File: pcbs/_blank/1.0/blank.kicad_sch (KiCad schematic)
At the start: 4 parts

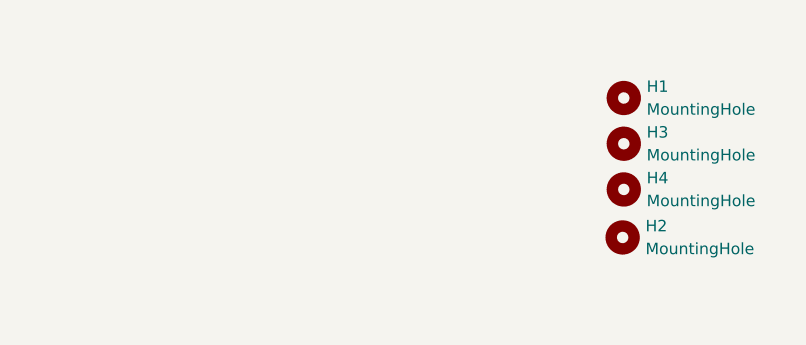
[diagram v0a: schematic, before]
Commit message: Staging
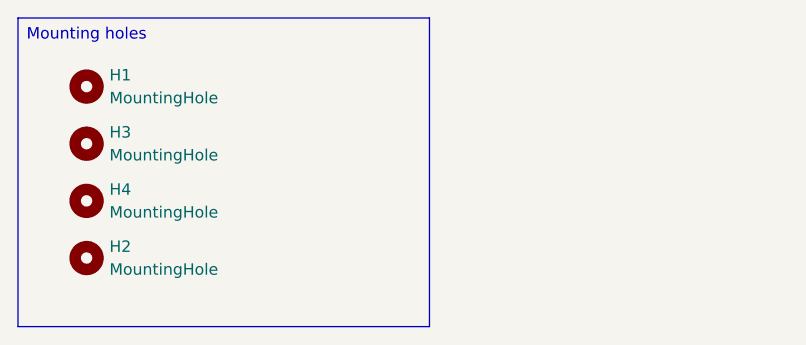
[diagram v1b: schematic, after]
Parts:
- H1, H2, H3, H4: footprint MountingHole:MountingHole_3.2mm_M3_DIN965_Pad_TopOnly -> MountingHole:MountingHole_3.2mm_M3_DIN965_Pad_TopBottom
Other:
- moved on the sheet: H1, H2, H3, H4
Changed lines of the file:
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@@
 (kicad_sch
-	(version 20231120)
+	(version 20250114)
 	(generator "eeschema")
-	(generator_version "8.0")
+	(generator_version "9.0")
 	(paper "A2")
-	(symbol
-		(lib_id "Mechanical:MountingHole")
-		(at 82.55 34.29 0)
+	(text_box "Mounting holes"
+		(exclude_from_sim no)
+		(at 15.24 15.24 0)
+		(size 45.72 34.29)
+		(margins 0.9525 0.9525 0.9525 0.9525)
+		(stroke
+			(width 0)
+			(type solid)
+		)
+		(fill
+			(type none)
+		)
+		(effects
+			(font
+				(size 1.27 1.27)
+			)
+			(justify left top)
+		)
+	)
+	(symbol
+		(lib_id "Mechanical:MountingHole")
+		(at 22.86 35.56 0)
 		(unit 1)
 		(exclude_from_sim no)
@@
 		(fields_autoplaced yes)
 		(property "Reference" "H4"
-			(at 85.09 33.0199 0)
-			(effects
-				(font
-					(size 1.27 1.27)
-				)
-				(justify left)
-			)
-		)
-		(property "Value" "MountingHole"
-			(at 85.09 35.5599 0)
-			(effects
-				(font
-					(size 1.27 1.27)
-				)
-				(justify left)
-			)
-		)
-		(property "Footprint" "MountingHole:MountingHole_3.2mm_M3_DIN965_Pad_TopOnly"
-			(at 82.55 34.29 0)
-			(effects
-				(font
-					(size 1.27 1.27)
-				)
-				(hide yes)
-			)
-		)
-		(property "Datasheet" "~"
-			(at 82.55 34.29 0)
-			(effects
-				(font
-					(size 1.27 1.27)
-				)
-				(hide yes)
-			)
-		)
-		(property "Description" ""
-			(at 82.55 34.29 0)
+			(at 25.4 34.2899 0)
+			(effects
+				(font
+					(size 1.27 1.27)
+				)
+				(justify left)
+			)
+		)
+		(property "Value" "MountingHole"
+			(at 25.4 36.8299 0)
+			(effects
+				(font
+					(size 1.27 1.27)
+				)
+				(justify left)
+			)
+		)
+		(property "Footprint" "MountingHole:MountingHole_3.2mm_M3_DIN965_Pad_TopBottom"
+			(at 22.86 35.56 0)
+			(effects
+				(font
+					(size 1.27 1.27)
+				)
+				(hide yes)
+			)
+		)
+		(property "Datasheet" "~"
+			(at 22.86 35.56 0)
+			(effects
+				(font
+					(size 1.27 1.27)
+				)
+				(hide yes)
+			)
+		)
+		(property "Description" ""
+			(at 22.86 35.56 0)
 			(effects
 				(font
@@
 	(symbol
 		(lib_id "Mechanical:MountingHole")
-		(at 82.55 29.21 0)
+		(at 22.86 29.21 0)
 		(unit 1)
 		(exclude_from_sim no)
@@
 		(fields_autoplaced yes)
 		(property "Reference" "H3"
-			(at 85.09 27.9399 0)
-			(effects
-				(font
-					(size 1.27 1.27)
-				)
-				(justify left)
-			)
-		)
-		(property "Value" "MountingHole"
-			(at 85.09 30.4799 0)
-			(effects
-				(font
-					(size 1.27 1.27)
-				)
-				(justify left)
-			)
-		)
-		(property "Footprint" "MountingHole:MountingHole_3.2mm_M3_DIN965_Pad_TopOnly"
-			(at 82.55 29.21 0)
-			(effects
-				(font
-					(size 1.27 1.27)
-				)
-				(hide yes)
-			)
-		)
-		(property "Datasheet" "~"
-			(at 82.55 29.21 0)
-			(effects
-				(font
-					(size 1.27 1.27)
-				)
-				(hide yes)
-			)
-		)
-		(property "Description" ""
-			(at 82.55 29.21 0)
+			(at 25.4 27.9399 0)
+			(effects
+				(font
+					(size 1.27 1.27)
+				)
+				(justify left)
+			)
+		)
+		(property "Value" "MountingHole"
+			(at 25.4 30.4799 0)
+			(effects
+				(font
+					(size 1.27 1.27)
+				)
+				(justify left)
+			)
+		)
+		(property "Footprint" "MountingHole:MountingHole_3.2mm_M3_DIN965_Pad_TopBottom"
+			(at 22.86 29.21 0)
+			(effects
+				(font
+					(size 1.27 1.27)
+				)
+				(hide yes)
+			)
+		)
+		(property "Datasheet" "~"
+			(at 22.86 29.21 0)
+			(effects
+				(font
+					(size 1.27 1.27)
+				)
+				(hide yes)
+			)
+		)
+		(property "Description" ""
+			(at 22.86 29.21 0)
 			(effects
 				(font
@@
 	(symbol
 		(lib_id "Mechanical:MountingHole")
-		(at 82.55 24.13 0)
+		(at 22.86 22.86 0)
 		(unit 1)
 		(exclude_from_sim no)
@@
 		(fields_autoplaced yes)
 		(property "Reference" "H1"
-			(at 85.09 22.8599 0)
-			(effects
-				(font
-					(size 1.27 1.27)
-				)
-				(justify left)
-			)
-		)
-		(property "Value" "MountingHole"
-			(at 85.09 25.3999 0)
-			(effects
-				(font
-					(size 1.27 1.27)
-				)
-				(justify left)
-			)
-		)
-		(property "Footprint" "MountingHole:MountingHole_3.2mm_M3_DIN965_Pad_TopOnly"
-			(at 82.55 24.13 0)
-			(effects
-				(font
-					(size 1.27 1.27)
-				)
-				(hide yes)
-			)
-		)
-		(property "Datasheet" "~"
-			(at 82.55 24.13 0)
-			(effects
-				(font
-					(size 1.27 1.27)
-				)
-				(hide yes)
-			)
-		)
-		(property "Description" ""
-			(at 82.55 24.13 0)
+			(at 25.4 21.5899 0)
+			(effects
+				(font
+					(size 1.27 1.27)
+				)
+				(justify left)
+			)
+		)
+		(property "Value" "MountingHole"
+			(at 25.4 24.1299 0)
+			(effects
+				(font
+					(size 1.27 1.27)
+				)
+				(justify left)
+			)
+		)
+		(property "Footprint" "MountingHole:MountingHole_3.2mm_M3_DIN965_Pad_TopBottom"
+			(at 22.86 22.86 0)
+			(effects
+				(font
+					(size 1.27 1.27)
+				)
+				(hide yes)
+			)
+		)
+		(property "Datasheet" "~"
+			(at 22.86 22.86 0)
+			(effects
+				(font
+					(size 1.27 1.27)
+				)
+				(hide yes)
+			)
+		)
+		(property "Description" ""
+			(at 22.86 22.86 0)
 			(effects
 				(font
@@
 	(symbol
 		(lib_id "Mechanical:MountingHole")
-		(at 82.423 39.624 0)
+		(at 22.86 41.91 0)
 		(unit 1)
 		(exclude_from_sim no)
@@
 		(fields_autoplaced yes)
 		(property "Reference" "H2"
-			(at 84.963 38.3539 0)
-			(effects
-				(font
-					(size 1.27 1.27)
-				)
-				(justify left)
-			)
-		)
-		(property "Value" "MountingHole"
-			(at 84.963 40.8939 0)
-			(effects
-				(font
-					(size 1.27 1.27)
-				)
-				(justify left)
-			)
-		)
-		(property "Footprint" "MountingHole:MountingHole_3.2mm_M3_DIN965_Pad_TopOnly"
-			(at 82.423 39.624 0)
-			(effects
-				(font
-					(size 1.27 1.27)
-				)
-				(hide yes)
-			)
-		)
-		(property "Datasheet" "~"
-			(at 82.423 39.624 0)
-			(effects
-				(font
-					(size 1.27 1.27)
-				)
-				(hide yes)
-			)
-		)
-		(property "Description" ""
-			(at 82.423 39.624 0)
+			(at 25.4 40.6399 0)
+			(effects
+				(font
+					(size 1.27 1.27)
+				)
+				(justify left)
+			)
+		)
+		(property "Value" "MountingHole"
+			(at 25.4 43.1799 0)
+			(effects
+				(font
+					(size 1.27 1.27)
+				)
+				(justify left)
+			)
+		)
+		(property "Footprint" "MountingHole:MountingHole_3.2mm_M3_DIN965_Pad_TopBottom"
+			(at 22.86 41.91 0)
+			(effects
+				(font
+					(size 1.27 1.27)
+				)
+				(hide yes)
+			)
+		)
+		(property "Datasheet" "~"
+			(at 22.86 41.91 0)
+			(effects
+				(font
+					(size 1.27 1.27)
+				)
+				(hide yes)
+			)
+		)
+		(property "Description" ""
+			(at 22.86 41.91 0)
 			(effects
 				(font
@@
 		)
 	)
+	(embedded_fonts no)
 )
